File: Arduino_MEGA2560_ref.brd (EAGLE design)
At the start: 66.7 x 104.8 mm, 80 parts, among them IC1 7805DT, IC2 7805DT, Q1 IRLML2502, Q10 PF610BL, Q11 IRLML2502, Q12 PF610BL, Q13 IRLML2502, Q14 PF610BL, Q2 PF610BL, Q3 IRLML2502, Q4 PF610BL, Q5 IRLML2502, Q6 PF610BL, Q7 IRLML2502, Q8 PF610BL, Q9 IRLML2502, X1 MKDSN1,5/2-5,08, X15 1751251, X16 1751251, X17 1751264, X2 MKDSN1,5/2-5,08, X3 MKDSN1,5/2-5,08, X4 MKDSN1,5/2-5,08, X5 MKDSN1,5/2-5,08, X6 MKDSN1,5/2-5,08, X7 5566-4, X8 1751248, X9 MKDSN1,5/2-5,08

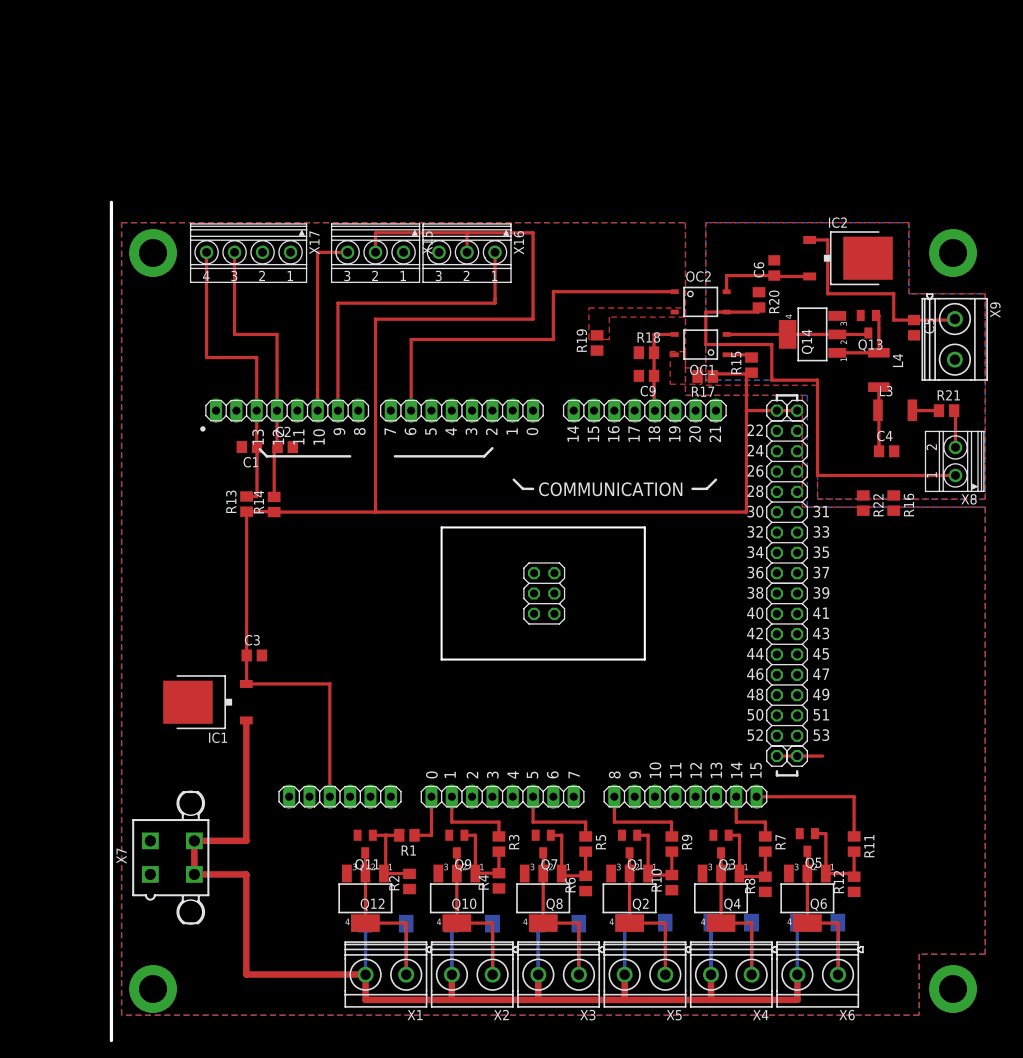
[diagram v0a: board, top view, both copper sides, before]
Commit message: doiing CAM
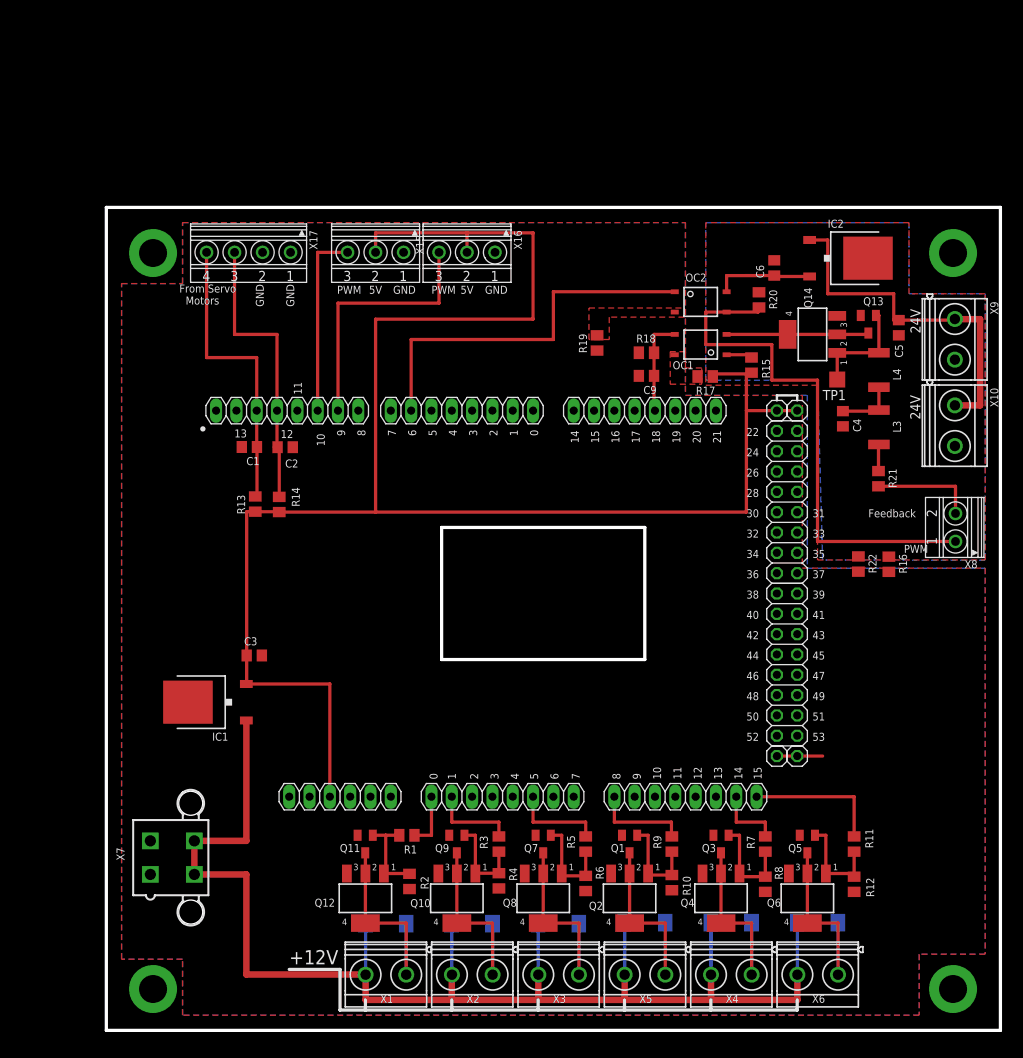
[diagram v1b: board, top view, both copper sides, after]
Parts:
- removed ICSP: ICSP, pinhead:2X03
- added TP1: PTR1TP20SQ, testpad:TP20SQ
- added X10: MKDSN1,5/2-5,08, con-phoenix-508:MKDSN1,5/2-5,08
- moved R21 12.0 mm to (106.7, 42.3), turned to 270 degrees
- moved X8 8.26 mm to (116.2, 36.2)
- moved R16 7.67 mm to (108.0, 31.6)
- moved R22 7.64 mm to (104.2, 31.6)
- moved C4 6.81 mm to (102.2, 49.8), turned to 270 degrees
- moved L3 2.95 mm to (106.7, 48.7), turned to 270 degrees
- moved C5 1.91 mm to (109.2, 61.2)
- moved R13 1.09 mm to (28.8, 39.1)
- moved R14 0.64 mm to (31.8, 39.1)
- moved Q5 0.20 mm to (97.8, -3.38)
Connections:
- net +24V: now also X10.1
- net GND: now also X16.1; no longer X16.3
- net GNDA: now also X10.2
- net N$21: now also TP1.TP
- net PH6: now also X16.3; no longer X16.1
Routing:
- net +24V: track 28.5 -> 45.5 mm
- net N$22: track 4.62 -> 13.0 mm
- net N$18: track 58.8 -> 67.0 mm
- net PH6: track 39.4 -> 32.4 mm
- net N$21: track 10.3 -> 13.6 mm
- net N$20: track 9.34 -> 7.49 mm
- net +5V: track 217.9 -> 216.6 mm
- net PB7: track 38.1 -> 37.0 mm
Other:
- board size 66.7 x 104.8 mm -> 111.8 x 102.9 mm
- board text added: "+12V"
- board text added: "24V"
- board text added: "5V"
- board text added: "Feedback"
- board text added: "From Servo Motors"
- board text added: "GND"
- board text added: "PWM"

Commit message: done factory
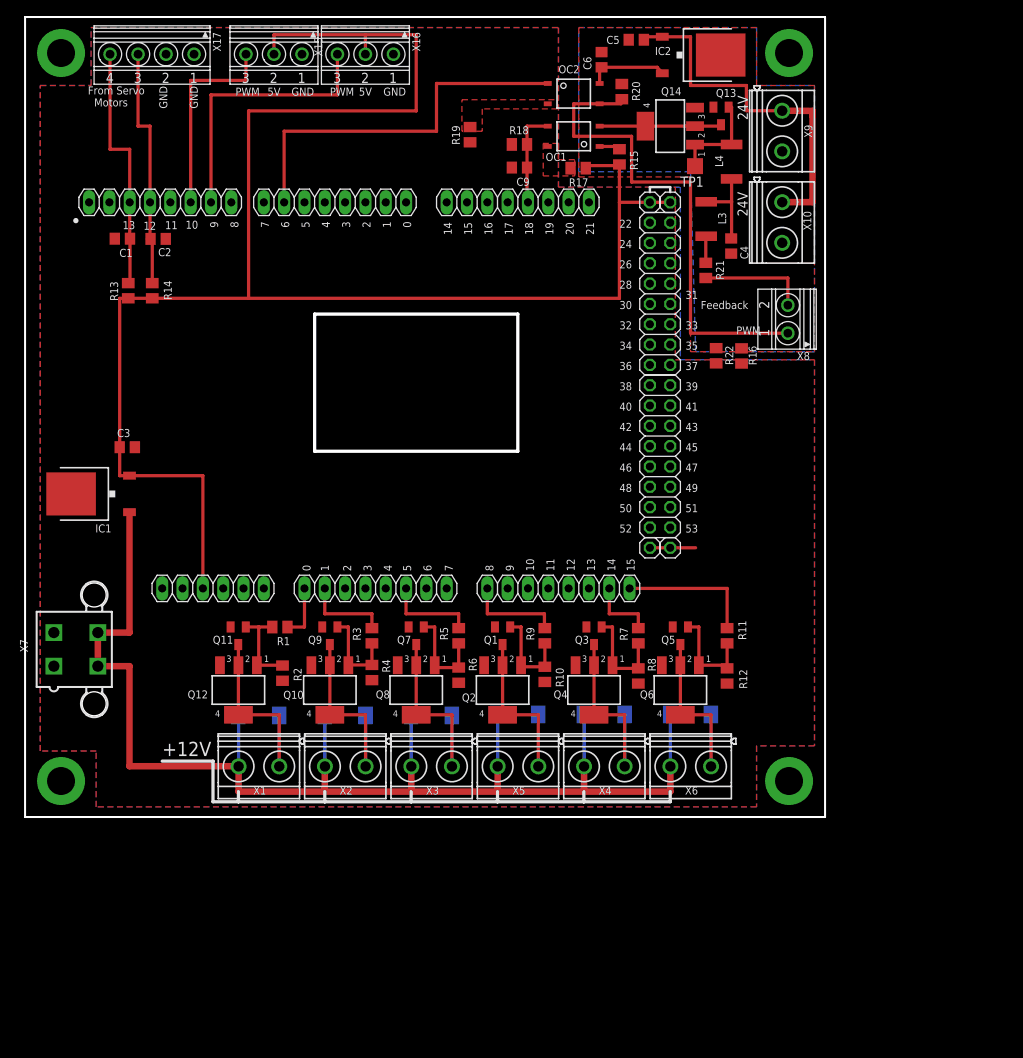
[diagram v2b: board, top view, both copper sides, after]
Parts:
- moved C5 48.7 mm to (76.4, 97.2), turned to 180 degrees
- moved C6 33.8 mm to (72.1, 94.7)
- moved L3 33.8 mm to (85.1, 74.8)
- moved R21 33.8 mm to (85.1, 68.3)
- moved X9 33.8 mm to (94.6, 85.7)
- moved X8 33.4 mm to (95.2, 62.2)
- moved X10 33.3 mm to (94.6, 74.3)
- moved TP1 32.1 mm to (83.7, 81.4)
- moved L4 31.9 mm to (88.3, 81.9)
- moved Q13 31.9 mm to (87.0, 87.6)
- moved R16 31.9 mm to (89.6, 57.6)
- moved R22 31.5 mm to (86.4, 57.7)
- moved Q14 31.5 mm to (80.6, 86.4)
- moved IC2 31.4 mm to (84.5, 95.2)
- moved R20 31.2 mm to (74.6, 90.7)
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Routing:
- net +12V: track 171.3 -> 165.0 mm
- net PB6: track 36.5 -> 30.8 mm
- net PB7: track 37.0 -> 31.3 mm
- net N$18: track 67.0 -> 61.9 mm
- net +5V: track 216.6 -> 213.3 mm
- net N$20: track 7.49 -> 10.7 mm
- net N$14: track 17.9 -> 15.3 mm
- net +5V_1: track 12.5 -> 10.3 mm
- net PH6: track 32.4 -> 34.3 mm
- net PB4: track 23.5 -> 25.4 mm
- net N$21: track 13.6 -> 12.3 mm
- net N$13: track 3.46 -> 2.82 mm
- net N$22: track 13.0 -> 13.7 mm
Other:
- board size 111.8 x 102.9 mm -> 100 x 100 mm
